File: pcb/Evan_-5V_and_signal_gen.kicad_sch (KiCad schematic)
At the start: 33 parts, among them IC1 TL7660IDGKR, IC2 TL081IDT, IC4 UA78M33CDCYG3, IC9 TL081IDT, U5 TPS2069CDBVR_MOSFET

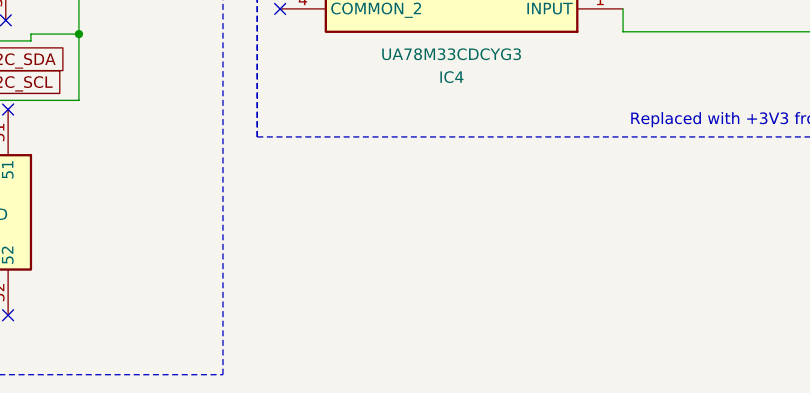
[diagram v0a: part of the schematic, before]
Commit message: Restructured PCB
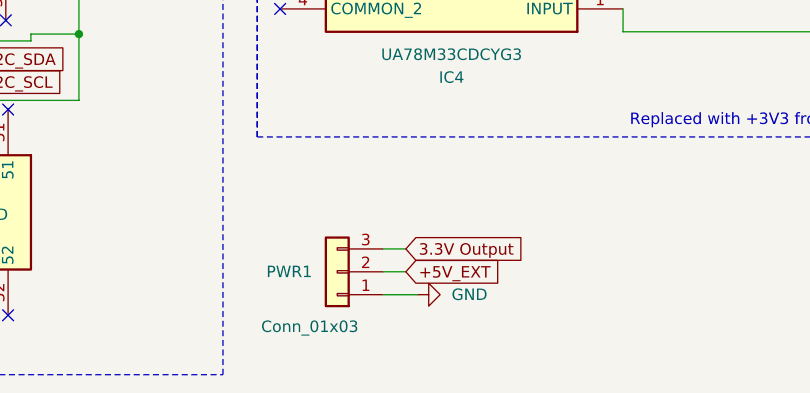
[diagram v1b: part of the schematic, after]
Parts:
- added PWR1: Conn_01x03, Connector_PinHeader_2.54mm:PinHeader_1x03_P2.54mm_Vertical, symbol Connector_Generic:Conn_01x03
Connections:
- net +5V_EXT: now also PWR1.2 (Pin_2)
- net 3.3V Output: now also PWR1.3 (Pin_3)
- net GND: now also PWR1.1 (Pin_1)
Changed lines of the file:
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@@
 	(wire
 		(pts
+			(xy 132.08 180.34) (xy 135.89 180.34)
+		)
+		(stroke
+			(width 0)
+			(type default)
+		)
+	)
+	(wire
+		(pts
 			(xy 208.28 97.79) (xy 208.28 101.6)
 		)
@@
 	(wire
 		(pts
+			(xy 132.08 175.26) (xy 134.62 175.26)
+		)
+		(stroke
+			(width 0)
+			(type default)
+		)
+	)
+	(wire
+		(pts
 			(xy 30.734 29.972) (xy 26.924 29.972)
 		)
@@
 	(wire
 		(pts
+			(xy 132.08 177.8) (xy 134.62 177.8)
+		)
+		(stroke
+			(width 0)
+			(type default)
+		)
+	)
+	(wire
+		(pts
 			(xy 172.72 38.1) (xy 187.96 38.1)
 		)
@@
 		)
 	)
+	(global_label "+5V_EXT"
+		(shape input)
+		(at 134.62 177.8 0)
+		(fields_autoplaced yes)
+		(effects
+			(font
+				(size 1.27 1.27)
+			)
+			(justify left)
+		)
+		(property "Intersheetrefs" "${INTERSHEET_REFS}"
+			(at 145.7694 177.8 0)
+			(effects
+				(font
+					(size 1.27 1.27)
+				)
+				(justify left)
+				(hide yes)
+			)
+		)
+	)
+	(global_label "3.3V Output"
+		(shape input)
+		(at 134.62 175.26 0)
+		(fields_autoplaced yes)
+		(effects
+			(font
+				(size 1.27 1.27)
+			)
+			(justify left)
+		)
+		(property "Intersheetrefs" "${INTERSHEET_REFS}"
+			(at 148.9141 175.26 0)
+			(effects
+				(font
+					(size 1.27 1.27)
+				)
+				(justify left)
+				(hide yes)
+			)
+		)
+	)
 	(symbol
 		(lib_id "capstone:T495D106K035ATE300")
@@
 	)
 	(symbol
+		(lib_id "Connector_Generic:Conn_01x03")
+		(at 127 177.8 180)
+		(unit 1)
+		(exclude_from_sim no)
+		(in_bom yes)
+		(on_board yes)
+		(dnp no)
+		(property "Reference" "PWR1"
+			(at 121.666 177.8 0)
+			(effects
+				(font
+					(size 1.27 1.27)
+				)
+			)
+		)
+		(property "Value" "Conn_01x03"
+			(at 123.952 183.896 0)
+			(effects
+				(font
+					(size 1.27 1.27)
+				)
+			)
+		)
+		(property "Footprint" "Connector_PinHeader_2.54mm:PinHeader_1x03_P2.54mm_Vertical"
+			(at 127 177.8 0)
+			(effects
+				(font
+					(size 1.27 1.27)
+				)
+				(hide yes)
+			)
+		)
+		(property "Datasheet" "~"
+			(at 127 177.8 0)
+			(effects
+				(font
+					(size 1.27 1.27)
+				)
+				(hide yes)
+			)
+		)
+		(property "Description" ""
+			(at 127 177.8 0)
+			(effects
+				(font
+					(size 1.27 1.27)
+				)
+				(hide yes)
+			)
+		)
+		(pin "1"
+		)
+		(pin "2"
+		)
+		(pin "3"
+		)
+		(instances
+			(project "mcu_integration"
+				(path "/c0210bc3-f67f-47d8-a34e-f002a728adb2/39708197-8fe0-4b5c-ba49-65ed06982da9"
+					(reference "PWR1")
+					(unit 1)
+				)
+			)
+		)
+	)
+	(symbol
 		(lib_name "GND_1")
 		(lib_id "power:GND")
@@
 					(unit 1)
 				)
+			)
+		)
+	)
+	(symbol
+		(lib_name "GND_4")
+		(lib_id "power:GND")
+		(at 135.89 180.34 90)
+		(unit 1)
+		(exclude_from_sim no)
+		(in_bom yes)
+		(on_board yes)
+		(dnp no)
+		(fields_autoplaced yes)
+		(property "Reference" "#PWR066"
+			(at 142.24 180.34 0)
+			(effects
+				(font
+					(size 1.27 1.27)
+				)
+				(hide yes)
+			)
+		)
+		(property "Value" "GND"
+			(at 139.7 180.3399 90)
+			(effects
+				(font
+					(size 1.27 1.27)
+				)
+				(justify right)
+			)
+		)
+		(property "Footprint" ""
+			(at 135.89 180.34 0)
+			(effects
+				(font
+					(size 1.27 1.27)
+				)
+				(hide yes)
+			)
+		)
+		(property "Datasheet" ""
+			(at 135.89 180.34 0)
+			(effects
+				(font
+					(size 1.27 1.27)
+				)
+				(hide yes)
+			)
+		)
+		(property "Description" "Power symbol creates a global label with name \"GND\" , ground"
+			(at 135.89 180.34 0)
+			(effects
+				(font
+					(size 1.27 1.27)
+				)
+				(hide yes)
+			)
+		)
+		(pin "1"
+		)
+		(instances
+			(project ""
+				(path "/c0210bc3-f67f-47d8-a34e-f002a728adb2/39708197-8fe0-4b5c-ba49-65ed06982da9"
+					(reference "#PWR066")
+					(unit 1)
+				)
